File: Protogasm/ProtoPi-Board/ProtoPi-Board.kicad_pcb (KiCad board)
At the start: 2 copper layers, 68.6 x 53.3 mm, 11 parts, among them J1 Neopixel_Ring_Header, J2 Jack-DC, M1 Motor_DC, Q1 FQP30N06L, SW1 Rotary_Encoder_Switch, U1 Arduino_UNO_R3, U2 MPX5050GP

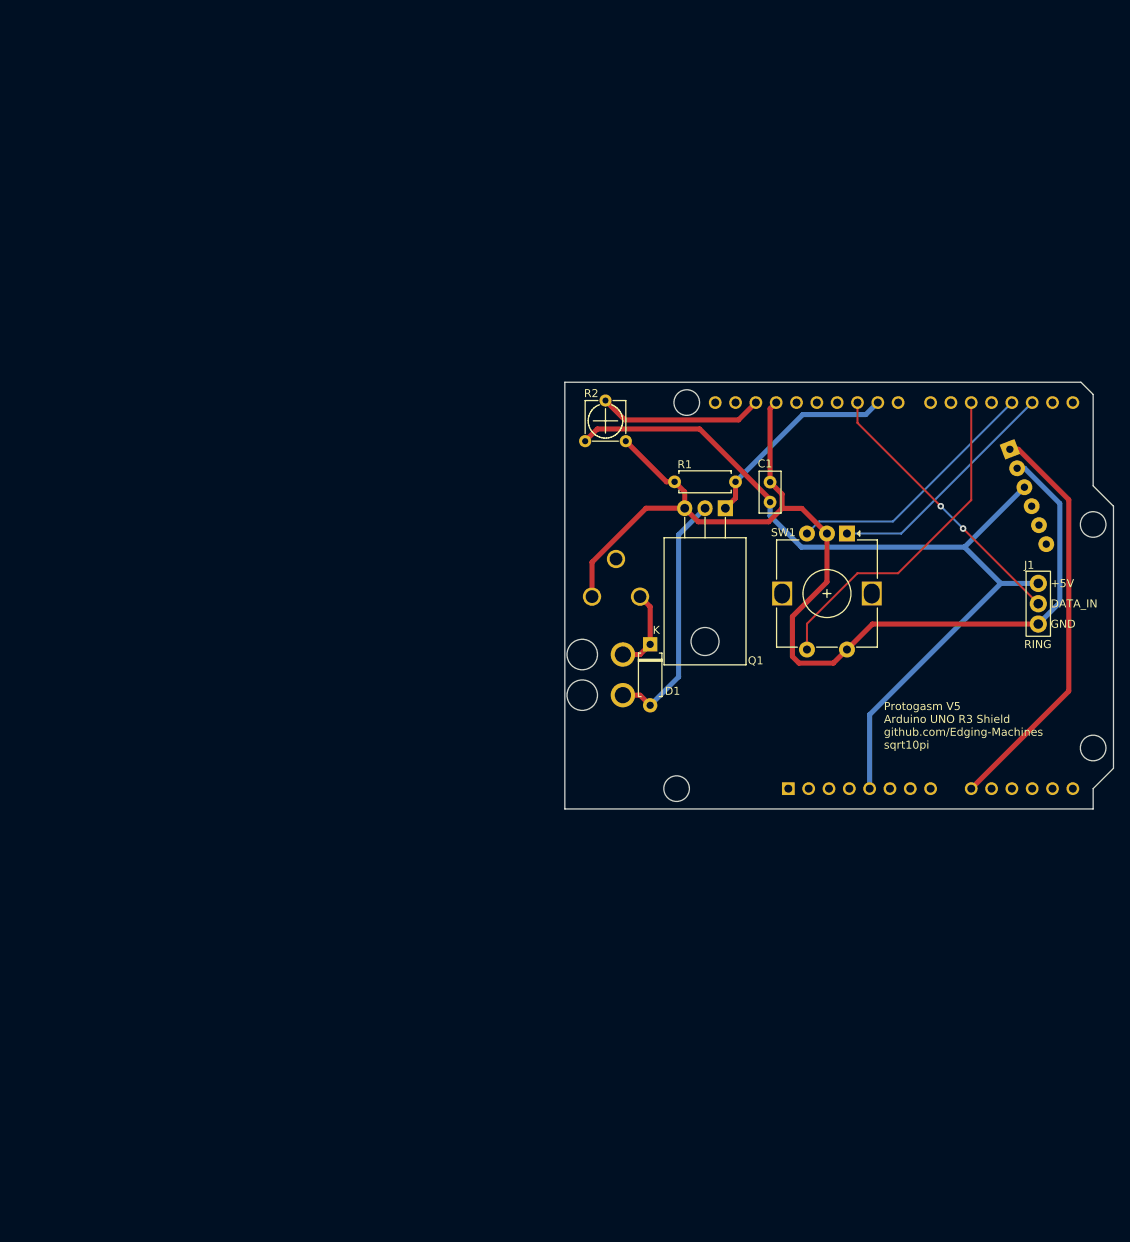
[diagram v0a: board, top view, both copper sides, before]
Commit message: v5
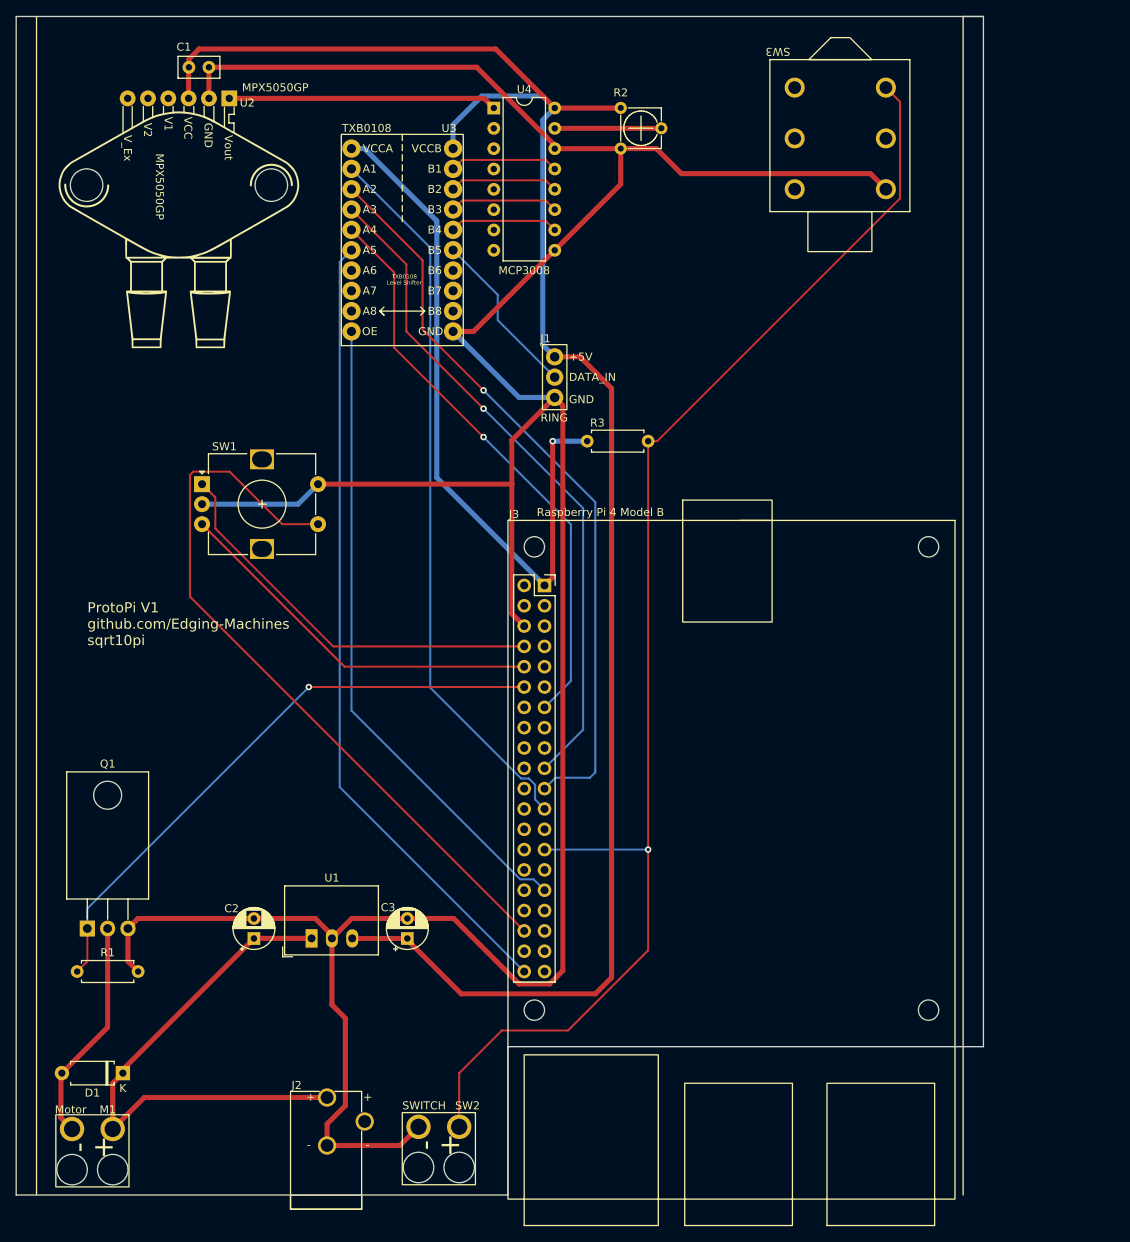
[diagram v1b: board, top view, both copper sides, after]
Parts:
- added C2: 10u, Capacitor_THT:CP_Radial_D5.0mm_P2.50mm, F.Cu at (70.4, 140.7)
- added C3: 10u, Capacitor_THT:CP_Radial_D5.0mm_P2.50mm, F.Cu at (89.5, 140.7)
- added J3: Raspberry_Pi_2_3, custom-footprints:Raspberry_Pi_4_Model_B, F.Cu at (150.6, 94.0)
- added R3: 2k, Resistor_THT:R_Axial_DIN0207_L6.3mm_D2.5mm_P7.62mm_Horizontal, F.Cu at (112.0, 78.5)
- added SW2: FOOTSWITCH, custom-footprints:Motor_DC_WirePins, F.Cu at (96.0, 164.2)
- added SW3: FOOTSWITCH (ALT), custom-footprints:CL1110, F.Cu at (149.4, 34.3)
- added U3: TXB0108, custom-footprints:TXB0108-Adafruit, F.Cu at (88.9, 53.3)
- added U4: MCP3008, Package_DIP:DIP-16_W7.62mm, F.Cu at (100.3, 36.8)
- J2, M1, U2: moved to F.Cu
- U1: value Arduino_UNO_R3 -> R-78E5.0-0.5; footprint Module:Arduino_UNO_R3_WithMountingHoles -> Converter_DCDC:Converter_DCDC_RECOM_R-78E-0.5_THT; moved to F.Cu
- moved U2 107.0 mm to (67.3, 35.6), turned to -90 degrees
- moved R1 102.6 mm to (48.3, 144.8), turned to 0 degrees
- moved Q1 95.5 mm to (49.5, 139.4), turned to 0 degrees
- moved C1 90.7 mm to (62.2, 31.8), turned to 0 degrees
- moved M1 87.1 mm to (52.7, 164.5), turned to -90 degrees
- moved D1 85.0 mm to (54.0, 157.5), turned to 180 degrees
- moved SW1 80.9 mm to (63.9, 83.9), turned to 0 degrees
- moved J2 73.8 mm to (79.5, 160.5), turned to 180 degrees
- moved J1 66.8 mm to (108.0, 67.9)
- moved U1 62.5 mm to (77.6, 140.6)
- moved R2 41.9 mm to (116.2, 36.8), turned to -90 degrees
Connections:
- J1 pad 2: /D10 -> /NEO_DATA_5V
- Q1 pad 1: /D9 -> /MOTOR_3V3
- R1 pad 1: /D9 -> /MOTOR_3V3
- R2 pad 2: /AREF -> /A_REF
- SW1 pad A: /D2 -> /SW_ROTA
- SW1 pad B: /D3 -> /SW_ROTB
- SW1 pad S2: /D5 -> /SW_PRESS
- U1 pad 1: unconnected-(U1-Pad1) -> +12V
- U1 pad 2: unconnected-(U1-Pad2) -> GND
- U1 pad 3: unconnected-(U1-Pad3) -> +5V
- U2 pad 1: /A0 -> /A_CH0
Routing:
- net GND: track 139.0 -> 394.6 mm
- net Net-(J3-Pad27): track 0.00 -> 171.9 mm, vias 0 -> 1
- net +5V: track 109.5 -> 231.3 mm
- net /NEO_DATA_3V3: track 0.00 -> 100.3 mm
- net /SW_PRESS: track 0.00 -> 93.2 mm
- net /MISO_3V3: track 0.00 -> 92.7 mm, vias 0 -> 1
- net /CLK_3V3: track 0.00 -> 90.6 mm
- net +3V3: track 0.00 -> 88.3 mm, vias 0 -> 1
- net /MOSI_3V3: track 0.00 -> 83.8 mm, vias 0 -> 1
- net /TXB_OE: track 0.00 -> 80.8 mm
- net /MOTOR_3V3: track 0.00 -> 74.5 mm, vias 0 -> 1
- net /~{CS_3V3}: track 0.00 -> 72.4 mm, vias 0 -> 1
- net +12V: track 10.8 -> 66.8 mm
- net /A0: track 51.1 -> 0.00 mm
- net /SW_ROTA: track 0.00 -> 50.9 mm
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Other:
- board size 68.6 x 53.3 mm -> 120.9 x 147.3 mm
- board text added: "MCP3008"
- board text added: "ProtoPi V1 github.com/Edging-Machines sqrt10pi"
- board text added: "Raspberry Pi 4 Model B"
- board text added: "TXB0108"
- board text removed: "12V 2A"
- board text removed: "Protogasm V5 Arduino UNO R3 Shield github.com/Edging-Machines sqrt10pi"
- board text removed: "crystal back side low clearance"
- board text removed: "tall"
- board text removed: "tall Arduino components no footprints on back side"
- board text removed: "tall components no footprints on back side"
